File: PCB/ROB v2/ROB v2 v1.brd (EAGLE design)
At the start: 100 x 62 mm, 15 parts, among them IC1 1182-A4988, IC2 1182-A4988, IC3 1182-A4988

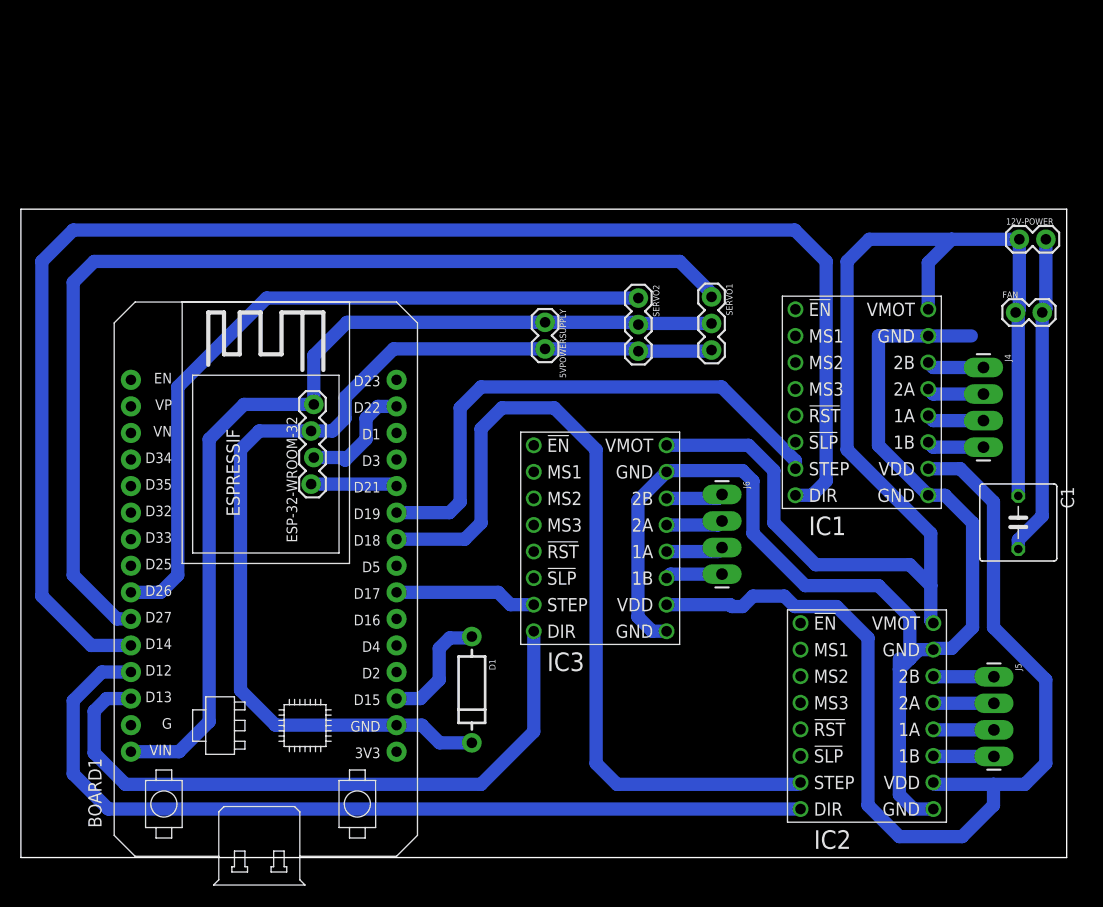
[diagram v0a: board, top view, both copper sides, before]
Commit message: updated schematics and board
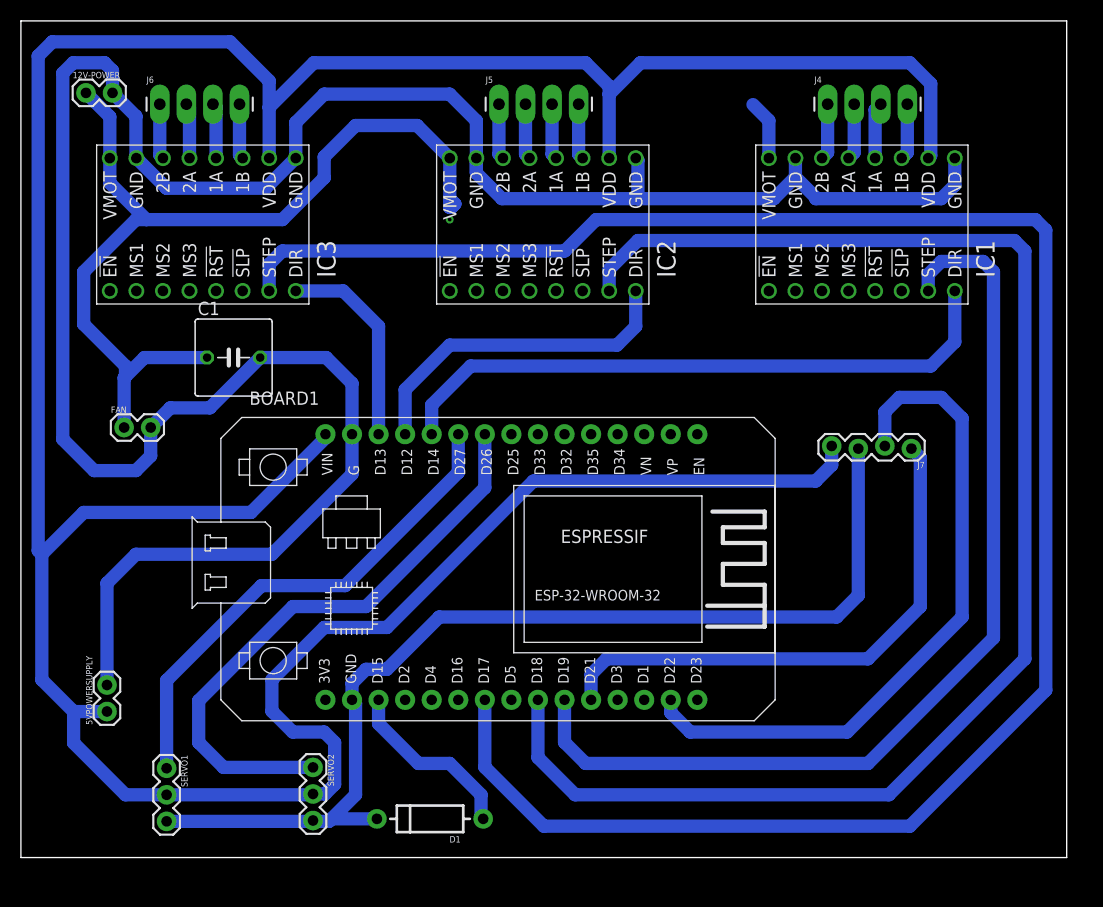
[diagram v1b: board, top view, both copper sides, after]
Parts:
- moved 12V-POWER 90.3 mm to (6.22, 73.1)
- moved FAN 86.0 mm to (9.87, 41.1)
- moved C1 76.7 mm to (20.3, 47.8), turned to 0 degrees
- moved J5 72.4 mm to (45.7, 72.0), turned to 0 degrees
- moved SERVO1 68.9 mm to (13.9, 8.54)
- moved J6 65.4 mm to (13.3, 72.0), turned to 0 degrees
- moved J7 57.4 mm to (85.2, 39.2), turned to 180 degrees
- moved IC2 56.3 mm to (49.9, 60.5), turned to 90 degrees
- moved 5VPOWERSUPPLY 56.0 mm to (8.23, 14.0), turned to 90 degrees
- moved SERVO2 54.6 mm to (27.9, 8.62)
- moved IC3 48.4 mm to (17.4, 60.5), turned to 90 degrees
- moved J4 29.3 mm to (77.1, 72.0), turned to 0 degrees
- moved IC1 17.0 mm to (80.4, 60.5), turned to 90 degrees
- moved D1 13.0 mm to (39.1, 3.70), turned to 180 degrees
- moved BOARD1 8.42 mm to (29.1, 15.1), turned to 0 degrees
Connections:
- net GND: now also BOARD1.GND
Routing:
- net STEP3: track 13.6 -> 190.8 mm
- net 5V: track 191.4 -> 321.7 mm
- net GND: track 249.5 -> 336.5 mm
- net DIR1: track 144.5 -> 60.2 mm
- net STEP2: track 81.7 -> 141.3 mm
- net SCL: track 11.3 -> 65.5 mm
- net DIR2: track 84.6 -> 32.2 mm
- net SIG2: track 98.7 -> 48.2 mm
- net SDA: track 8.25 -> 52.1 mm
- net DIR3: track 63.0 -> 19.6 mm
- net STEP1: track 52.1 -> 94.6 mm
- net 12V: track 121.5 -> 94.7 mm
- net SIG1: track 70.7 -> 56.8 mm
- net LED: track 11.4 -> 17.3 mm
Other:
- board size 100 x 62 mm -> 100 x 80 mm
